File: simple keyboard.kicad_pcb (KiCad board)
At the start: 2 copper layers, 81 x 28 mm, 19 parts, among them J1 USB_C_Receptacle_USB2.0_14P, SW1 SW_Push, SW2 SW_Push, SW3 SW_Push, U1 ATtiny25-20P

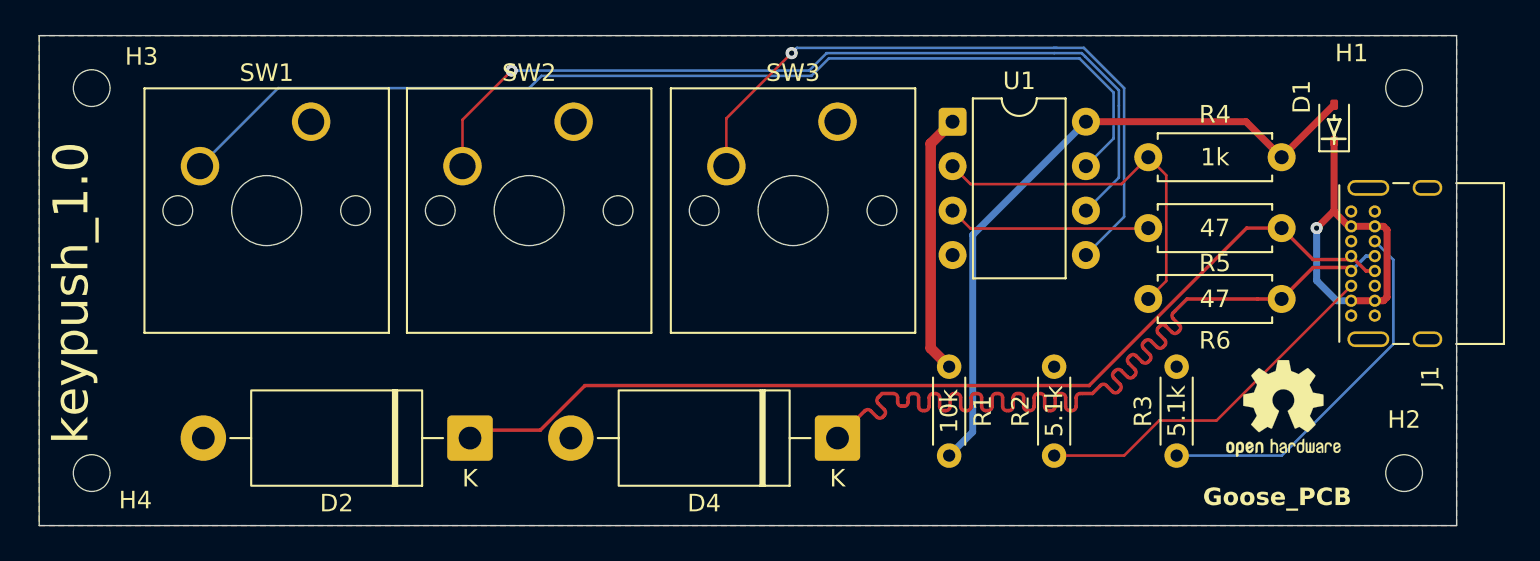
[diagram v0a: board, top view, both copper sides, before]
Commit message: updata 29 3 26
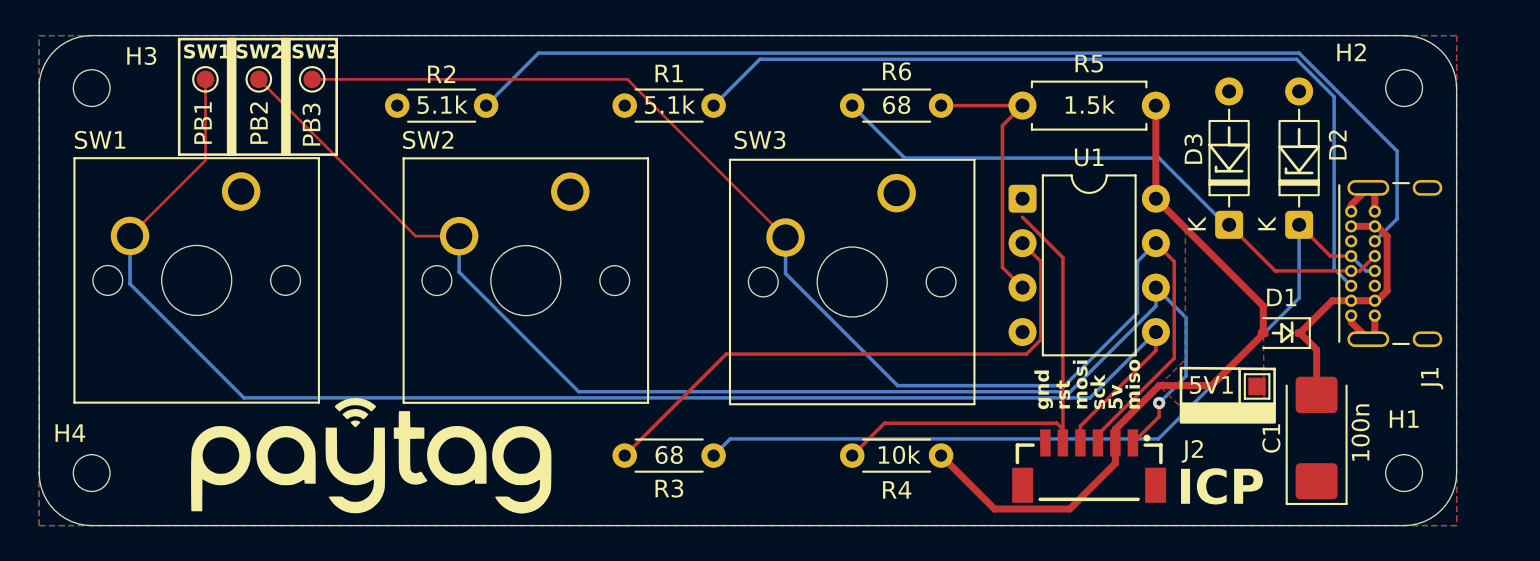
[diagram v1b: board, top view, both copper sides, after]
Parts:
- removed D4: 1N53xxB, Diode_THT:D_DO-201_P15.24mm_Horizontal
- removed REF**: OSHW-Logo2_7.3x6mm_SilkScreen, Symbol:OSHW-Logo2_7.3x6mm_SilkScreen
- added 5V1: TestPoint, TestPoint:TestPoint_Pad_1.0x1.0mm, F.Cu at (229.6, 40.0)
- added C1: 100n, Capacitor_Tantalum_SMD:CP_EIA-6032-28_Kemet-C, F.Cu at (233.0, 43.0)
- added D3: 3.6V, Diode_THT:D_DO-35_SOD27_P7.62mm_Horizontal, F.Cu at (228.0, 30.8)
- added G***: LOGO, Symbol:paytag logo, F.Cu at (179.0, 44.0)
- added J2: AVR-ISP-6, 665306124022:665306124022, F.Cu at (220.0, 45.0)
- added PB1: TestPoint, TestPoint:TestPoint_Pad_D1.0mm, F.Cu at (169.5, 22.5)
- added PB2: TestPoint, TestPoint:TestPoint_Pad_D1.0mm, F.Cu at (172.6, 22.5)
- added PB3: TestPoint, TestPoint:TestPoint_Pad_D1.0mm, F.Cu at (175.6, 22.5)
- D2: value 1N53xxB -> 3.6V; footprint Diode_THT:D_DO-201_P15.24mm_Horizontal -> Diode_THT:D_DO-35_SOD27_P7.62mm_Horizontal
- R1: value 10k -> 5.1k
- R3: value 5.1k -> 68
- R4: value 1k -> 10k; footprint Resistor_THT:R_Axial_DIN0207_L6.3mm_D2.5mm_P7.62mm_Horizontal -> Resistor_THT:R_Axial_DIN0204_L3.6mm_D1.6mm_P5.08mm_Horizontal
- R5: value 47 -> 1.5k
- R6: value 47 -> 68; footprint Resistor_THT:R_Axial_DIN0207_L6.3mm_D2.5mm_P7.62mm_Horizontal -> Resistor_THT:R_Axial_DIN0204_L3.6mm_D1.6mm_P5.08mm_Horizontal
- U1: value ATtiny25-20P -> ATtiny85-20P
- moved D2 48.9 mm to (232.0, 30.8), turned to 90 degrees
- moved R2 38.1 mm to (185.5, 24.0), turned to 180 degrees
- moved R4 29.9 mm to (206.5, 44.0), turned to 0 degrees
- moved R6 26.9 mm to (206.5, 24.0), turned to 0 degrees
- moved R3 26.5 mm to (198.5, 44.0), turned to 180 degrees
- moved R1 20.1 mm to (198.5, 24.0), turned to 180 degrees
- moved R5 16.4 mm to (216.2, 24.0), turned to 0 degrees
- moved D1 12.4 mm to (231.0, 37.0), turned to 180 degrees
- moved U1 5.95 mm to (216.2, 29.3)
- moved SW1 5.65 mm to (171.5, 28.9)
- moved SW3 5.30 mm to (209.0, 29.0)
- moved SW2 4.00 mm to (190.3, 28.9)
- renumbered H2 to H1, H1 to H2
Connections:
- net /s1 renamed /PB1
- D2 pad 1: /D- -> Net-(D2-K)
- J1 pad A6: /D+ -> Net-(D3-K)
- J1 pad A7: /D- -> Net-(D2-K)
- J1 pad B6: /D+ -> Net-(D3-K)
- J1 pad B7: /D- -> Net-(D2-K)
- R1 pad 1: /rst -> /CC1
- R1 pad 2: /5V -> GND
- R2 pad 1: /CC1 -> /CC2
- R3 pad 1: /CC2 -> Net-(D2-K)
- R3 pad 2: GND -> /D-
- R4 pad 1: /5V -> /PB5
- R4 pad 2: /xtal1 -> /5V
- R5 pad 1: /D- -> /D+
- R5 pad 2: /xtal2 -> /5V
- R6 pad 1: /D+ -> Net-(D3-K)
- R6 pad 2: /xtal1 -> /D+
- SW1 pad 2: /s2 -> /PB0
- SW3 pad 2: /s0 -> /PB2
- U1 pad 1: /rst -> /PB5
- U1 pad 2: /xtal1 -> /D-
- U1 pad 3: /xtal2 -> /D+
- U1 pad 5: /s0 -> /PB0
- U1 pad 7: /s2 -> /PB2
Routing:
- net /PB0: track 0.00 -> 84.5 mm
- net /PB2: track 0.00 -> 75.4 mm
- net /s2: track 60.4 -> 0.00 mm
- net Net-(D2-K): track 0.00 -> 46.8 mm
- net /D+: track 57.2 -> 16.0 mm
- net /CC2: track 21.3 -> 61.3 mm
- net /s0: track 38.5 -> 0.00 mm, vias 1 -> 0
- net Net-(D3-K): track 0.00 -> 34.1 mm
- net /CC1: track 21.0 -> 48.7 mm
- net /PB5: track 0.00 -> 27.6 mm
- net /D-: track 57.9 -> 32.5 mm
- net /PB1: track 50.3 -> 73.8 mm
- net /xtal1: track 21.2 -> 0.00 mm
- net /rst: track 15.0 -> 0.00 mm
- net /xtal2: track 11.6 -> 0.00 mm
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- added copper zone on F.Cu, net /5V
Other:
- outline, holes or cut-outs redrawn
- board text added: "5v"
- board text added: "ICP"
- board text added: "SW1"
- board text added: "SW2"
- board text added: "SW3"
- board text added: "gnd"
- board text added: "miso"
- board text added: "mosi"
- board text added: "rst"
- board text added: "sck"
- board text removed: "Goose_PCB"
- board text removed: "keypush_1.0"
